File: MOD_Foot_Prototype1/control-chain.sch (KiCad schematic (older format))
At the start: 24 parts, among them J1 RJ45_CHAIN, J2 RJ45_CHAIN, Q1 MMBT3904, Q2 MMBT3904, U1 SN75176BDR

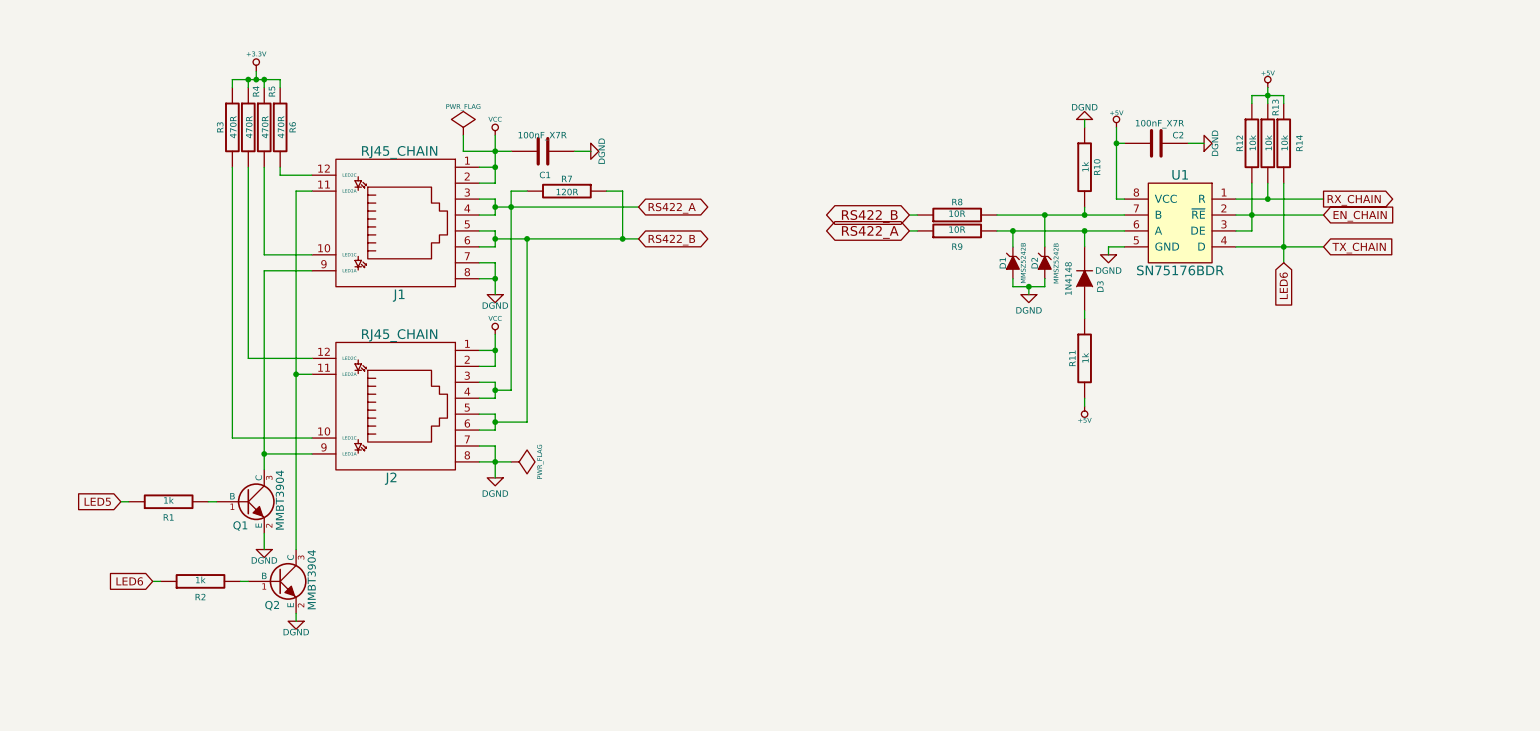
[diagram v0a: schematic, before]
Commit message: fix issue #4: sch: full duplex control chain circuit done
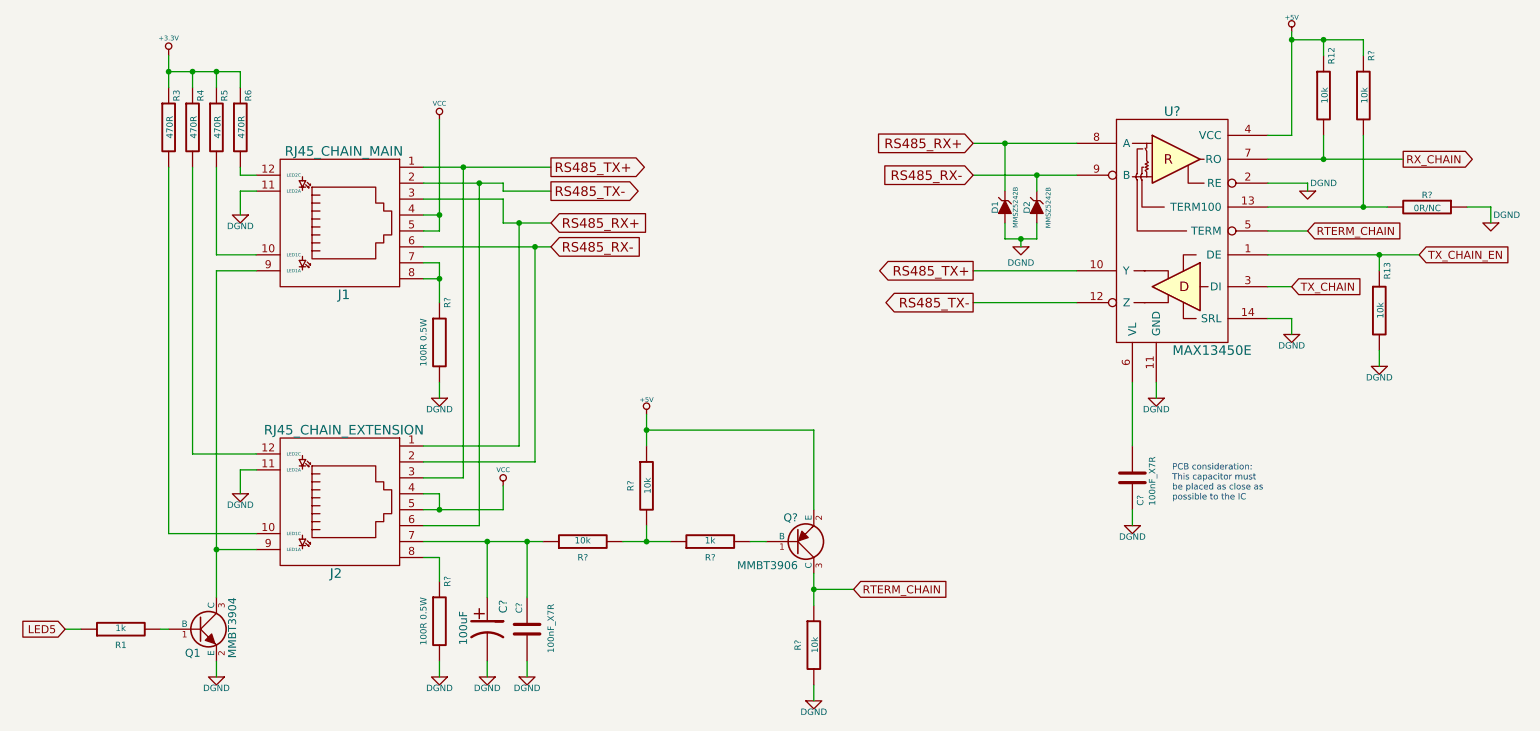
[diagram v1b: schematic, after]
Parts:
- removed C1, C2: 100nF_X7R, MOD_Footprints_Lib:SM0603, symbol C
- removed D3: 1N4148, MOD_Footprints_Lib:SOD323, symbol DIODE
- removed Q2: MMBT3904, MOD_Footprints_Lib:SOT23, symbol NPN
- removed R10, R11, R2: 1k, MOD_Footprints_Lib:SM0603, symbol R
- removed R14: 10k, MOD_Footprints_Lib:SM0603, symbol R
- removed R7: 120R, MOD_Footprints_Lib:SM0805, symbol R
- removed R8, R9: 10R, MOD_Footprints_Lib:SM0805, symbol R
- removed U1: SN75176BDR, MOD_Footprints_Lib:SO8E, symbol SN75176BDR
- added C? (x2): 100nF_X7R, MOD_Footprints_Lib:SM0603, symbol C
- added C?: 100uF, MOD_Footprints_Lib:CAP_RAD_5MM, symbol CP1
- added Q?: MMBT3906, symbol MMBT3906
- added R? (x4): 10k, MOD_Footprints_Lib:SM0603, symbol R
- added R?: 0R/NC, MOD_Footprints_Lib:SM0805, symbol R
- added R? (x2): 100R 0.5W, symbol R
- added R?: 1k, MOD_Footprints_Lib:SM0603, symbol R
- added U?: MAX13450E, TSSOP-14EP, symbol MAX13450E
- J1: value RJ45_CHAIN -> RJ45_CHAIN_MAIN
- J2: value RJ45_CHAIN -> RJ45_CHAIN_EXTENSION
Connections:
- net EN_CHAIN is gone; now on net RX_CHAIN: R12.2
- net +5V: now also Q?.2 (E), R?.1, R?.1, U?.4 (VCC); no longer R13.1
- net DGND: now also J1.11 (LED2A), J2.11 (LED2A), R13.2, C?.2, C?.2, C?.2, R?.1, R?.2, R?.2, R?.2, U?.11 (GND), U?.14 (SRL), U?.2 (RE); no longer J1.7, J1.8, J2.7, J2.8
- net RX_CHAIN: now also U?.7 (RO); no longer R13.2
- net VCC: now also J1.4, J1.5, J2.4, J2.5; no longer J1.1, J1.2, J2.1, J2.2
- net RS485_RX+: now reaches D1.2 (K)
- net RS485_RX+: now also J1.3, J2.1, U?.8 (A)
- net RS485_RX-: now reaches D2.2 (K)
- net RS485_RX-: now also J1.6, J2.2, U?.9 (B)
- removed net RS422_A: J1.3, J1.4, J2.3, J2.4
- removed net RS422_B: J1.5, J1.6, J2.5, J2.6
- new net: J1.7, J1.8, R?.1
- new net: C?.1, C?.1, J2.7, R?.1
- new net: J2.8, R?.1
- new net: R?.2, R?.2, U?.13 (TERM100)
- new net: C?.1, U?.6 (VL)
- new net: R?.1, R?.2, R?.2
- new net: Q?.1 (B), R?.2
- new net RS485_TX+: J1.1, J2.3, U?.10 (Y)
- new net RS485_TX-: J1.2, J2.6, U?.12 (Z)
- new net RTERM_CHAIN: Q?.3 (C), R?.1, U?.5 (TERM)
- new net TX_CHAIN: U?.3 (DI)
- new net TX_CHAIN_EN: R13.1, U?.1 (DE)
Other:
- note added: "PCB consideration: \nThis capacitor must \nbe placed as close as \npossible to the IC"
- moved on the sheet: D1, D2, J1, J2, Q1, R1, R12, R13, R3, R4, R5, R6
